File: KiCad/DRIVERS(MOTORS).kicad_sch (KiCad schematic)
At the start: 15 parts, among them M1 Motor_DC, M2 Motor_DC, M3 Motor_DC, U1 TB6612FNG, U2 TB6612FNG, U3 TB6612FNG

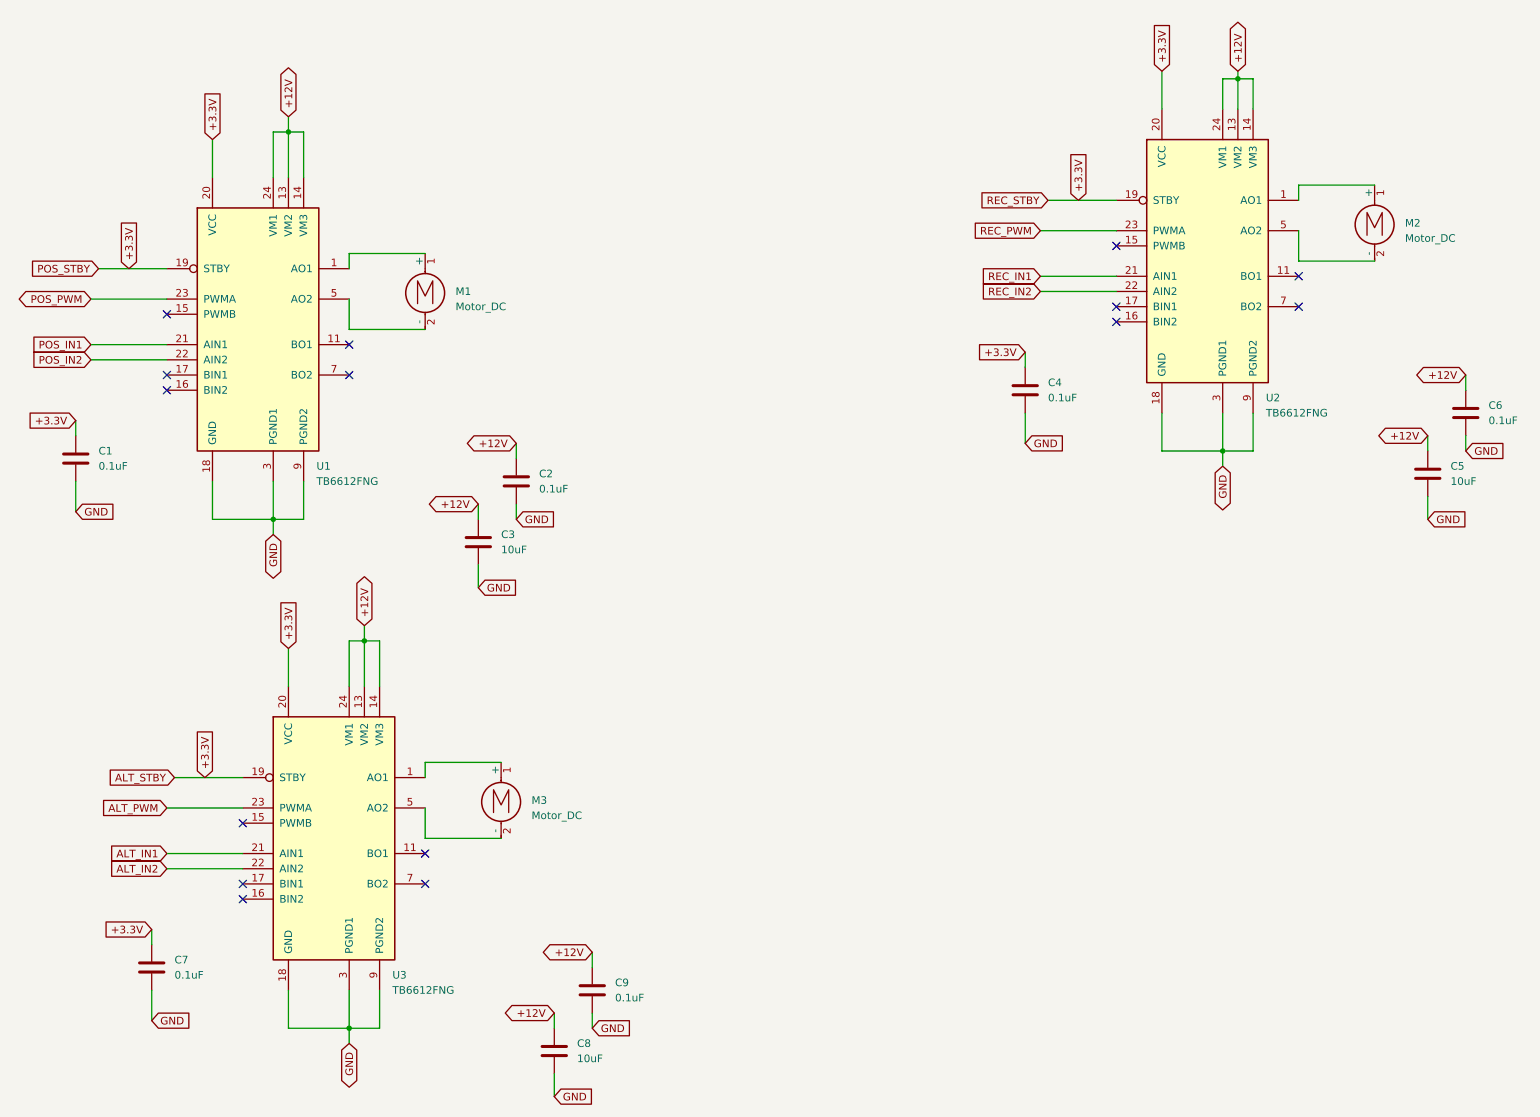
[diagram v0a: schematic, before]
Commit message: Canvis al KICAD
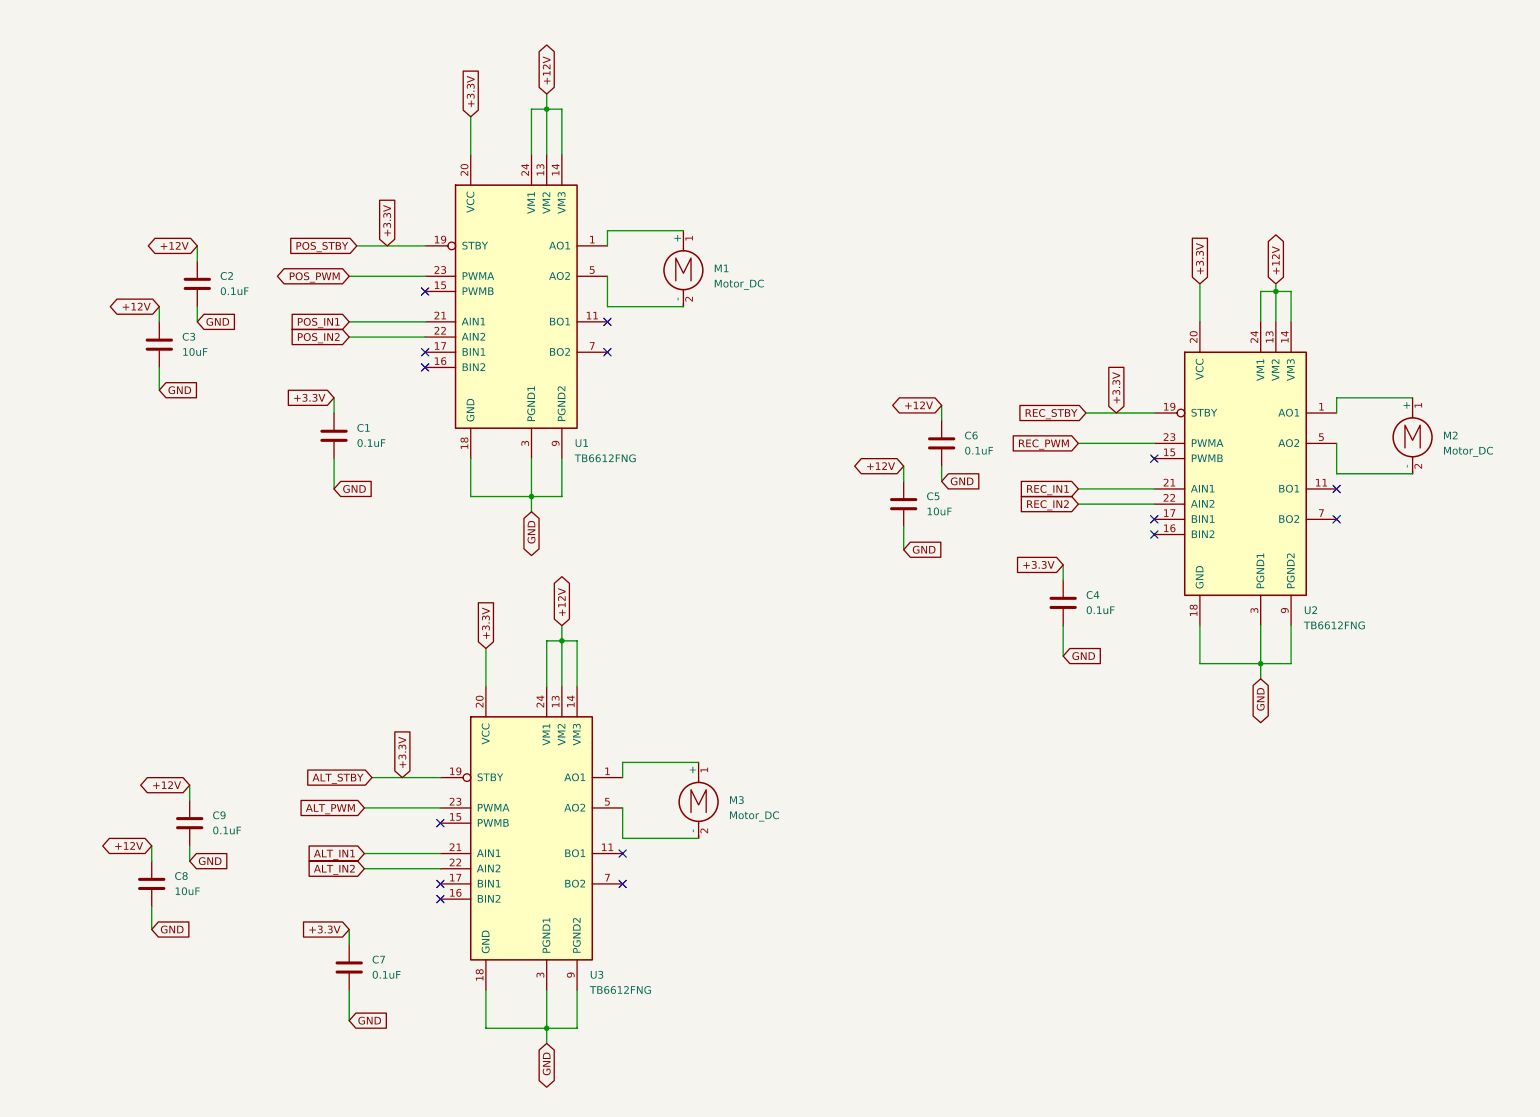
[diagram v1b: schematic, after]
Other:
- moved on the sheet: C1, C2, C3, C4, C5, C6, C7, C8, C9, M1, M2, M3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
